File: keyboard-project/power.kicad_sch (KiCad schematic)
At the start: 0 parts

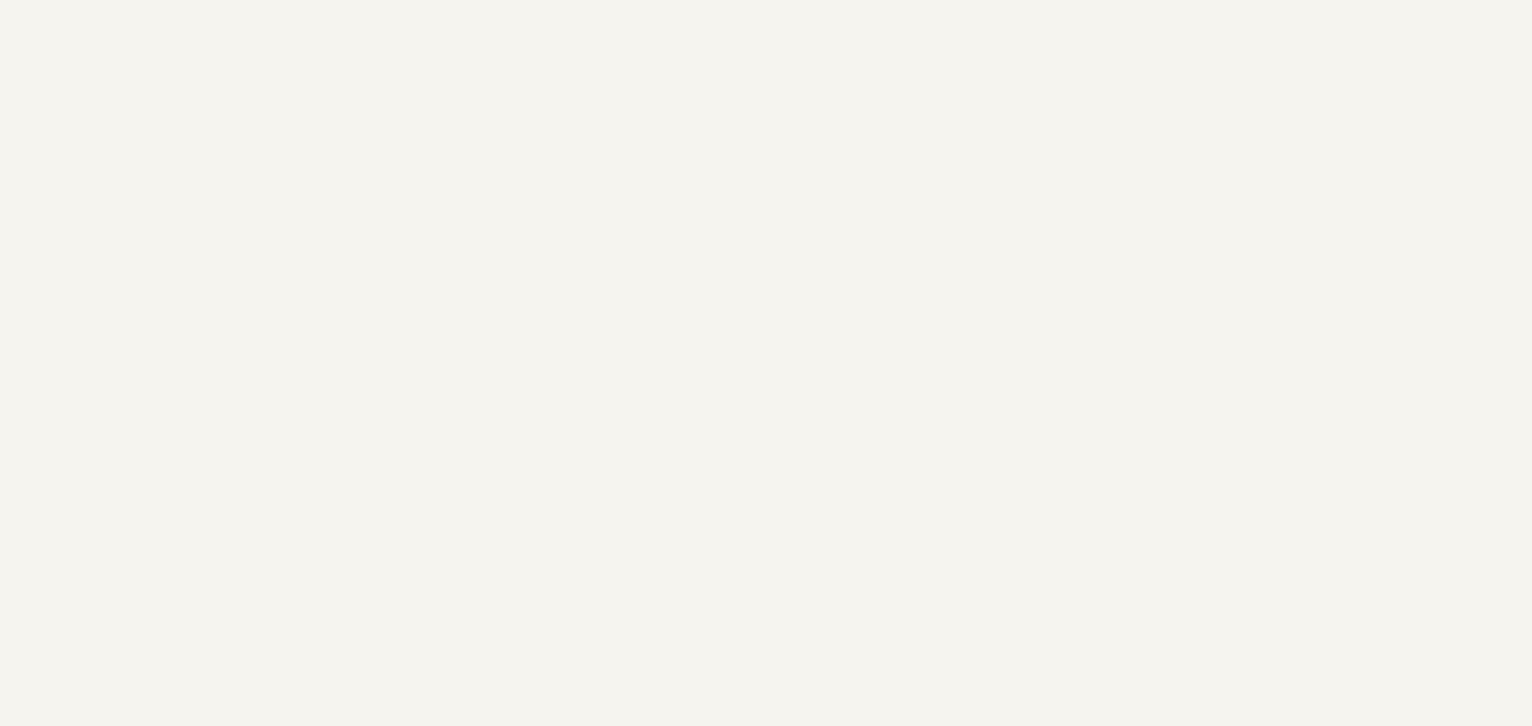
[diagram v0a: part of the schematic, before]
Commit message: working on power
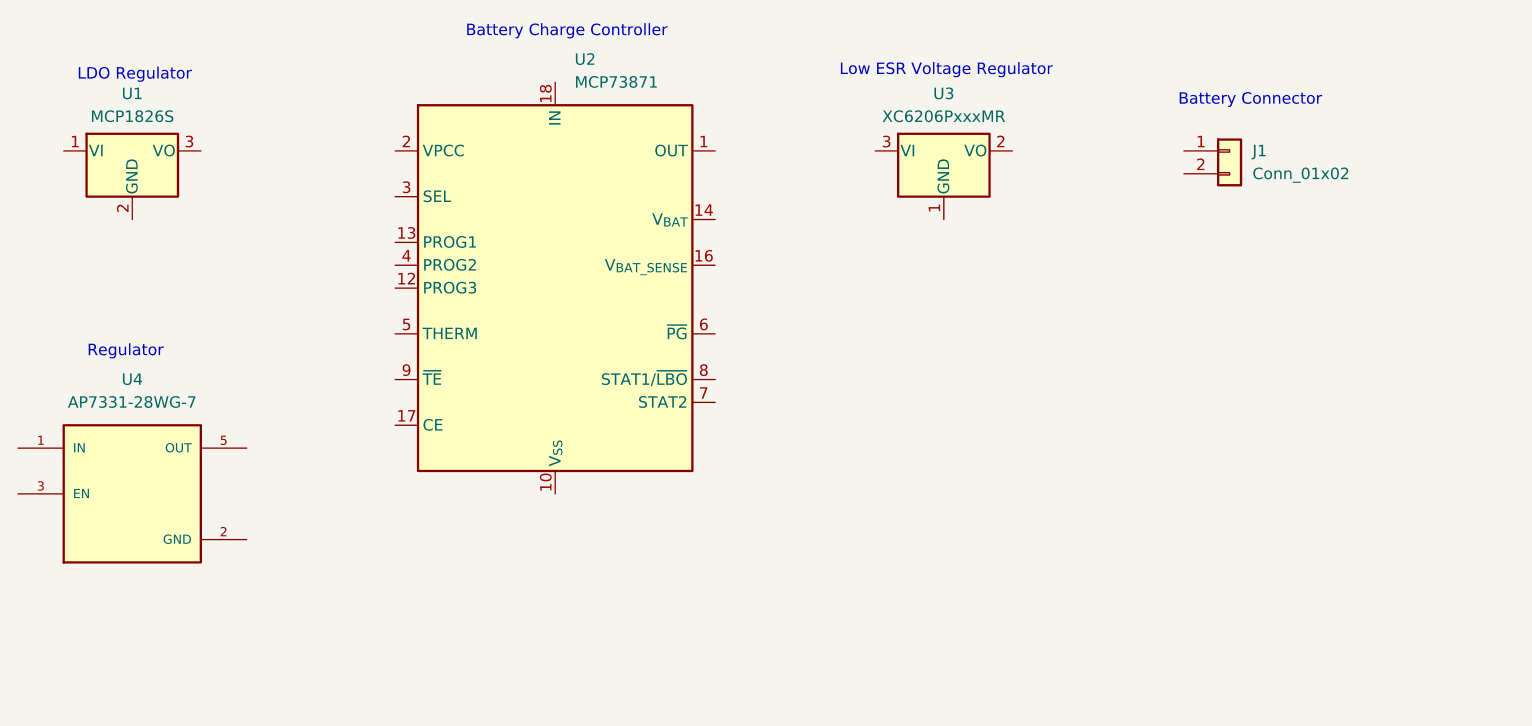
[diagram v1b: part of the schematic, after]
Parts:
- added J1: Conn_01x02, symbol Connector_Generic:Conn_01x02
- added U1: MCP1826S, symbol Regulator_Linear:MCP1826S
- added U2: MCP73871, Package_DFN_QFN:QFN-20-1EP_4x4mm_P0.5mm_EP2.5x2.5mm, symbol Battery_Management:MCP73871
- added U3: XC6206PxxxMR, Package_TO_SOT_SMD:SOT-23-3, symbol Regulator_Linear:XC6206PxxxMR
- added U4: AP7331-28WG-7, AP7331-28WG-7:SOT95P285X145-5N, symbol AP7331-28WG-7:AP7331-28WG-7
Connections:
- new net: U2.1 (OUT), U2.20 (OUT)
- new net: U2.10 (V_{SS}), U2.11 (V_{SS}), U2.21 (V_{SS})
- new net: U2.14 (V_{BAT}), U2.15 (V_{BAT})
- new net: U2.18 (IN), U2.19 (IN)
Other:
- note added: "Battery Charge Controller"
- note added: "Battery Connector"
- note added: "LDO Regulator"
- note added: "Low ESR Voltage Regulator"
- note added: "Regulator"
